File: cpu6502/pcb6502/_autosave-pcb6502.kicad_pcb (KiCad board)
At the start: 2 copper layers, 135.9 x 95.3 mm, 42 parts, among them J1 Power, J2 RS232, J3 VIA, J4 Reset Ext, J5 Boot, J6 Ext Pwr Sw, J8 RS232 CTS, SW1 Reset, SW2 Interrupts, U1 6502 (CPU), U2 28C256 (ROM), U3 62256 (RAM), U4 6522 (VIA), U5 74HC00, U6 L7805, U7 6551 (ACIA), U8 MAX232, U9 DS1813, X1 1MHz, Y1 1.8432 Mhz

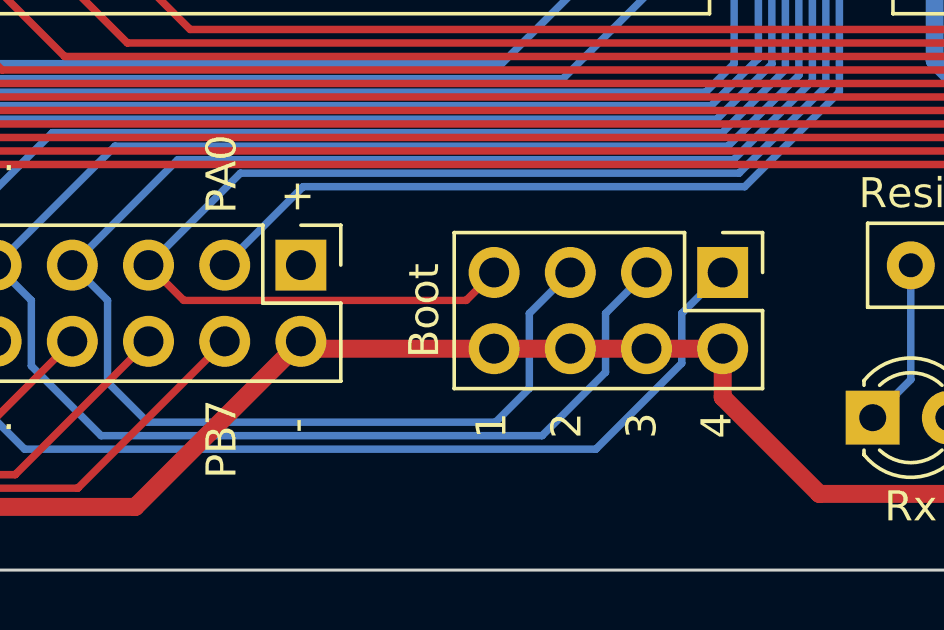
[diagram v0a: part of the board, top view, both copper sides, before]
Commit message: more basic progs
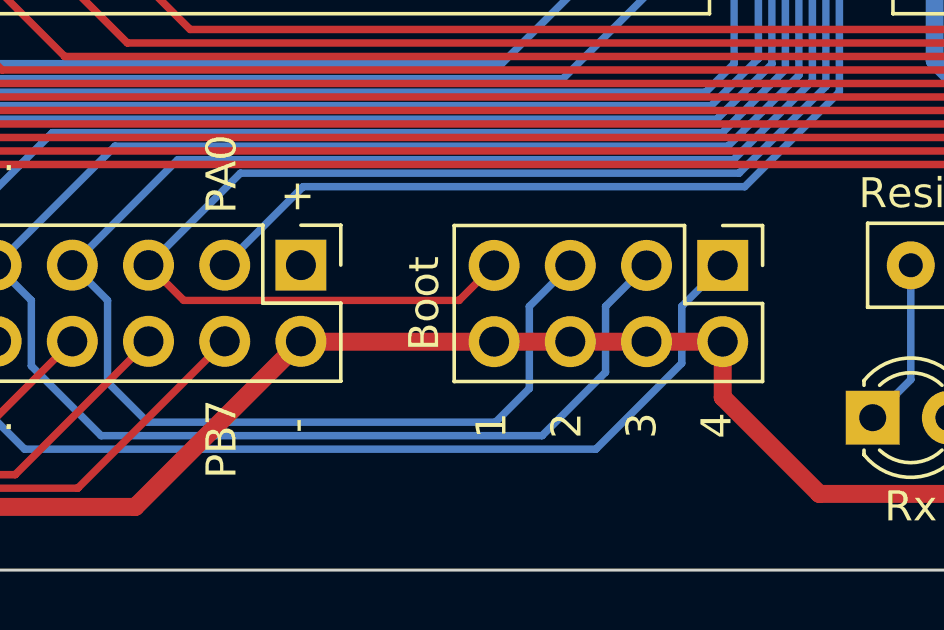
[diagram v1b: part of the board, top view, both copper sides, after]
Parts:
- moved J5 0.23 mm to (129.6, 109.2)
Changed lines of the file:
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@@
 	(footprint "Connector_PinHeader_2.54mm:PinHeader_2x04_P2.54mm_Vertical"
 		(layer "F.Cu")
-		(at 129.62 109.46 -90)
+		(at 129.62 109.225 -90)
 		(descr "Through hole straight pin header, 2x04, 2.54mm pitch, double rows")
 		(tags "Through hole pin header THT 2x04 2.54mm double row")
@@
 	)
 	(segment
+		(start 132.84 116.84)
+		(end 129.62 113.62)
+		(width 0.6)
+		(layer "F.Cu")
+		(net 28)
+	)
+	(segment
 		(start 165.5 115.5)
 		(end 152.33 115.5)
@@
 	)
 	(segment
+		(start 148.59 116.84)
+		(end 132.84 116.84)
+		(width 0.6)
+		(layer "F.Cu")
+		(net 28)
+	)
+	(segment
 		(start 169.705495 53.79)
 		(end 173.99 49.505495)
@@
 	)
 	(segment
+		(start 129.62 113.62)
+		(end 129.62 111.765)
+		(width 0.6)
+		(layer "F.Cu")
+		(net 28)
+	)
+	(segment
 		(start 97.5 35)
 		(end 97.5 32.09)
@@
 	)
 	(segment
-		(start 115.805 112)
-		(end 115.56 111.755)
-		(width 0.6)
-		(layer "F.Cu")
-		(net 28)
-	)
-	(segment
 		(start 169.816828 53.79)
 		(end 169.705495 53.79)
@@
 	)
 	(segment
-		(start 132.84 116.84)
-		(end 129.62 113.62)
-		(width 0.6)
-		(layer "F.Cu")
-		(net 28)
-	)
-	(segment
 		(start 89 48.31)
 		(end 85.69 48.31)
@@
 	)
 	(segment
-		(start 129.62 112)
-		(end 122 112)
-		(width 0.6)
-		(layer "F.Cu")
-		(net 28)
-	)
-	(segment
 		(start 97 48.31)
 		(end 93 48.31)
@@
 	)
 	(segment
-		(start 148.59 116.84)
-		(end 132.84 116.84)
-		(width 0.6)
-		(layer "F.Cu")
-		(net 28)
-	)
-	(segment
 		(start 173.99 33.02)
 		(end 179.41 27.6)
@@
 	)
 	(segment
-		(start 122 112)
-		(end 115.805 112)
-		(width 0.6)
-		(layer "F.Cu")
-		(net 28)
-	)
-	(segment
 		(start 85.69 48.31)
 		(end 76 58)
@@
 	)
 	(segment
-		(start 129.62 113.62)
-		(end 129.62 112)
+		(start 115.57 111.765)
+		(end 115.56 111.755)
+		(width 0.6)
+		(layer "F.Cu")
+		(net 28)
+	)
+	(segment
+		(start 129.62 111.765)
+		(end 115.57 111.765)
 		(width 0.6)
 		(layer "F.Cu")
@@
 	)
 	(segment
-		(start 122 109.46)
-		(end 121.07 110.39)
+		(start 120.835 110.39)
+		(end 111.655 110.39)
 		(width 0.25)
 		(layer "F.Cu")
@@
 	)
 	(segment
-		(start 121.07 110.39)
-		(end 111.655 110.39)
+		(start 122 109.225)
+		(end 120.835 110.39)
 		(width 0.25)
 		(layer "F.Cu")
@@
 	)
 	(segment
-		(start 124.54 109.46)
-		(end 123.175 110.825)
+		(start 109.115 113.115)
+		(end 109.115 110.39)
+		(width 0.25)
+		(layer "B.Cu")
+		(net 86)
+	)
+	(segment
+		(start 122.05 114.45)
+		(end 110.45 114.45)
 		(width 0.25)
 		(layer "B.Cu")
@@
 	)
 	(segment
-		(start 120.46698 84.265)
-		(end 132.61 96.40802)
+		(start 123.175 113.325)
+		(end 122.05 114.45)
 		(width 0.25)
 		(layer "B.Cu")
@@
 	)
 	(segment
-		(start 129.98198 105.7)
-		(end 111.455 105.7)
+		(start 120.46698 84.265)
+		(end 132.61 96.40802)
 		(width 0.25)
 		(layer "B.Cu")
@@
 	)
 	(segment
-		(start 111.455 105.7)
-		(end 107.94 109.215)
+		(start 129.98198 105.7)
+		(end 111.455 105.7)
 		(width 0.25)
 		(layer "B.Cu")
@@
 	)
 	(segment
-		(start 109.115 113.115)
-		(end 109.115 110.39)
+		(start 123.175 110.59)
+		(end 123.175 113.325)
 		(width 0.25)
 		(layer "B.Cu")
@@
 	)
 	(segment
-		(start 109.115 110.39)
+		(start 111.455 105.7)
 		(end 107.94 109.215)
 		(width 0.25)
@@
 	)
 	(segment
-		(start 123.175 113.325)
-		(end 122.05 114.45)
+		(start 109.115 110.39)
+		(end 107.94 109.215)
 		(width 0.25)
 		(layer "B.Cu")
@@
 	)
 	(segment
-		(start 123.175 110.825)
-		(end 123.175 113.325)
+		(start 110.45 114.45)
+		(end 109.115 113.115)
 		(width 0.25)
 		(layer "B.Cu")
@@
 	)
 	(segment
-		(start 110.45 114.45)
-		(end 109.115 113.115)
-		(width 0.25)
-		(layer "B.Cu")
-		(net 86)
-	)
-	(segment
-		(start 122.05 114.45)
-		(end 110.45 114.45)
+		(start 124.54 109.225)
+		(end 123.175 110.59)
 		(width 0.25)
 		(layer "B.Cu")
@@
 	)
 	(segment
-		(start 108.9 114.9)
-		(end 106.575 112.575)
+		(start 125.715 112.785)
+		(end 123.6 114.9)
 		(width 0.25)
 		(layer "B.Cu")
@@
 	)
 	(segment
+		(start 123.6 114.9)
+		(end 108.9 114.9)
+		(width 0.25)
+		(layer "B.Cu")
+		(net 88)
+	)
+	(segment
 		(start 129.465584 93.9)
 		(end 132.16 96.594416)
@@
 	)
 	(segment
-		(start 123.6 114.9)
-		(end 108.9 114.9)
+		(start 127.08 109.225)
+		(end 125.715 110.59)
 		(width 0.25)
 		(layer "B.Cu")
@@
 	)
 	(segment
-		(start 125.715 110.825)
-		(end 125.715 112.785)
+		(start 106.575 110.39)
+		(end 105.4 109.215)
 		(width 0.25)
 		(layer "B.Cu")
@@
 	)
 	(segment
-		(start 125.715 112.785)
-		(end 123.6 114.9)
+		(start 125.715 110.59)
+		(end 125.715 112.785)
 		(width 0.25)
 		(layer "B.Cu")
@@
 	)
 	(segment
-		(start 106.575 110.39)
-		(end 105.4 109.215)
+		(start 106.575 112.575)
+		(end 106.575 110.39)
 		(width 0.25)
 		(layer "B.Cu")
@@
 	)
 	(segment
-		(start 127.08 109.46)
-		(end 125.715 110.825)
-		(width 0.25)
-		(layer "B.Cu")
-		(net 88)
-	)
-	(segment
-		(start 106.575 112.575)
-		(end 106.575 110.39)
+		(start 108.9 114.9)
+		(end 106.575 112.575)
 		(width 0.25)
 		(layer "B.Cu")
@@
 	)
 	(segment
-		(start 125.391701 115.35)
-		(end 106.350001 115.35)
+		(start 106.350001 115.35)
+		(end 104.035 113.034999)
 		(width 0.25)
 		(layer "B.Cu")
@@
 	)
 	(segment
-		(start 128.255 110.825)
-		(end 128.255 112.486701)
+		(start 129.609188 104.8)
+		(end 107.275 104.8)
 		(width 0.25)
 		(layer "B.Cu")
@@
 	)
 	(segment
-		(start 129.609188 104.8)
-		(end 107.275 104.8)
+		(start 131.71 96.780812)
+		(end 131.71 102.699188)
 		(width 0.25)
 		(layer "B.Cu")
@@
 	)
 	(segment
-		(start 104.035 110.39)
-		(end 102.86 109.215)
+		(start 104.035 113.034999)
+		(end 104.035 110.39)
 		(width 0.25)
 		(layer "B.Cu")
@@
 	)
 	(segment
-		(start 131.71 96.780812)
-		(end 131.71 102.699188)
+		(start 115.090495 84.265)
+		(end 125.175495 94.35)
 		(width 0.25)
 		(layer "B.Cu")
@@
 	)
 	(segment
-		(start 115.090495 84.265)
-		(end 125.175495 94.35)
+		(start 104.035 110.39)
+		(end 102.86 109.215)
 		(width 0.25)
 		(layer "B.Cu")
@@
 	)
 	(segment
-		(start 129.62 109.46)
-		(end 128.255 110.825)
+		(start 125.391701 115.35)
+		(end 106.350001 115.35)
 		(width 0.25)
 		(layer "B.Cu")
@@
 	)
 	(segment
-		(start 107.275 104.8)
-		(end 102.86 109.215)
+		(start 129.62 109.225)
+		(end 128.255 110.59)
 		(width 0.25)
 		(layer "B.Cu")
@@
 	)
 	(segment
-		(start 131.71 102.699188)
-		(end 129.609188 104.8)
+		(start 107.275 104.8)
+		(end 102.86 109.215)
 		(width 0.25)
 		(layer "B.Cu")
@@
 	)
 	(segment
-		(start 106.350001 115.35)
-		(end 104.035 113.034999)
+		(start 128.255 110.59)
+		(end 128.255 112.486701)
 		(width 0.25)
 		(layer "B.Cu")
@@
 	)
 	(segment
-		(start 125.175495 94.35)
-		(end 129.279188 94.35)
+		(start 131.71 102.699188)
+		(end 129.609188 104.8)
 		(width 0.25)
 		(layer "B.Cu")
@@
 	)
 	(segment
-		(start 104.035 113.034999)
-		(end 104.035 110.39)
+		(start 125.175495 94.35)
+		(end 129.279188 94.35)
 		(width 0.25)
 		(layer "B.Cu")
